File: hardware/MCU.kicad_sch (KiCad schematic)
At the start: 12 parts

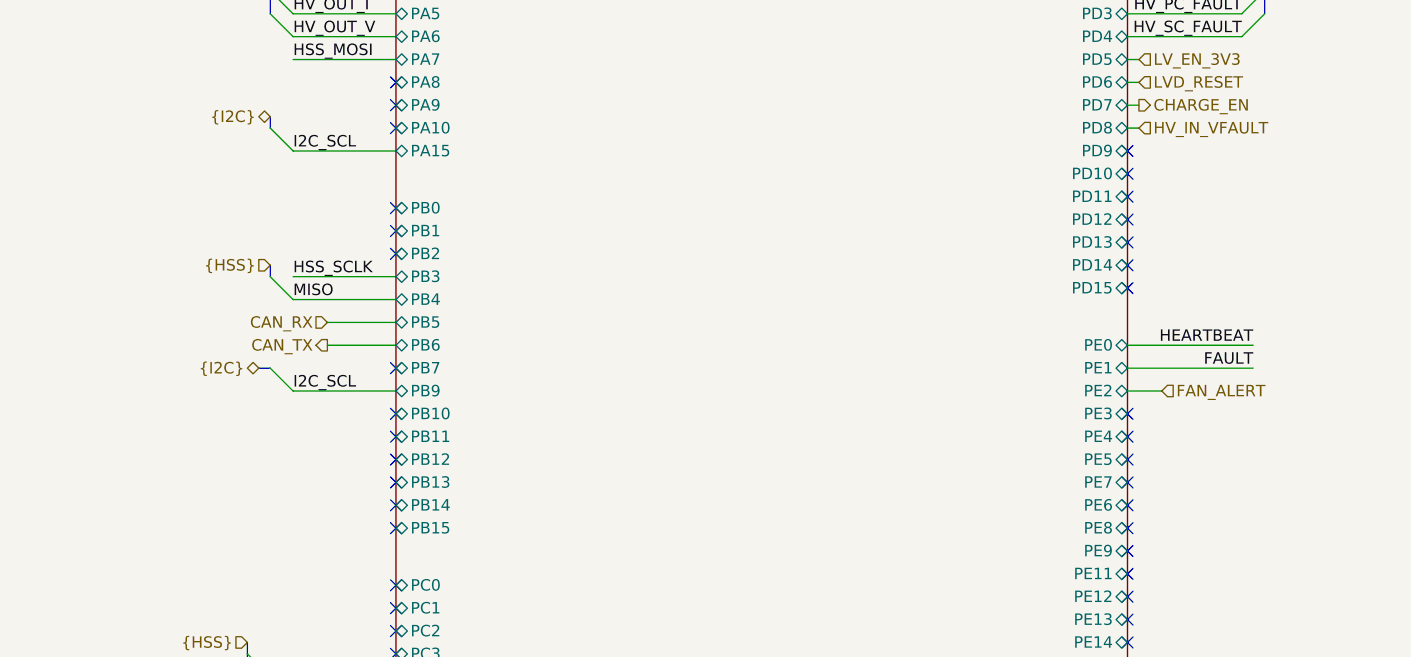
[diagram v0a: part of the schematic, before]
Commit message: review me pt 3
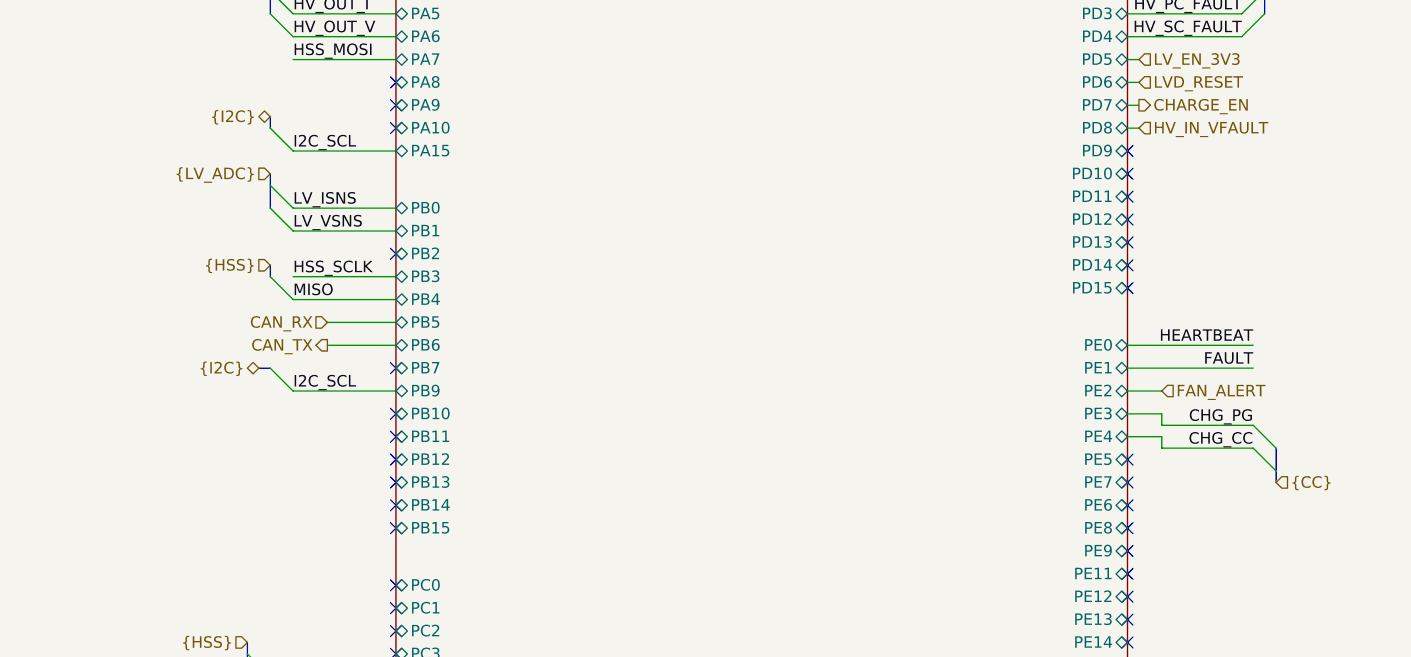
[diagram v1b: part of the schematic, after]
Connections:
- no-connect marks 49 -> 45
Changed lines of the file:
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@@
 	)
 	(no_connect
-		(at 287.02 90.17)
-	)
-	(no_connect
 		(at 287.02 154.94)
 	)
 	(no_connect
-		(at 368.3 110.49)
-	)
-	(no_connect
 		(at 287.02 78.74)
 	)
@@
 	)
 	(no_connect
-		(at 368.3 113.03)
-	)
-	(no_connect
 		(at 368.3 133.35)
 	)
@@
 		(at 368.3 149.86)
 	)
-	(no_connect
-		(at 287.02 87.63)
-	)
 	(bus_entry
 		(at 383.54 63.5)
@@
 	)
 	(bus_entry
+		(at 273.05 85.09)
+		(size 2.54 2.54)
+		(stroke
+			(width 0)
+			(type default)
+		)
+	)
+	(bus_entry
 		(at 273.05 95.25)
 		(size 2.54 2.54)
@@
 	)
 	(bus_entry
+		(at 384.81 114.3)
+		(size -2.54 -2.54)
+		(stroke
+			(width 0)
+			(type default)
+		)
+	)
+	(bus_entry
 		(at 273.05 63.5)
 		(size 2.54 2.54)
@@
 	)
 	(bus_entry
+		(at 273.05 87.63)
+		(size 2.54 2.54)
+		(stroke
+			(width 0)
+			(type default)
+		)
+	)
+	(bus_entry
 		(at 273.05 58.42)
 		(size 2.54 2.54)
@@
 	)
 	(bus_entry
+		(at 384.81 116.84)
+		(size -2.54 -2.54)
+		(stroke
+			(width 0)
+			(type default)
+		)
+	)
+	(bus_entry
 		(at 270.51 137.16)
 		(size 2.54 2.54)
@@
 	(wire
 		(pts
+			(xy 372.11 114.3) (xy 382.27 114.3)
+		)
+		(stroke
+			(width 0)
+			(type default)
+		)
+	)
+	(wire
+		(pts
 			(xy 368.3 73.66) (xy 369.57 73.66)
 		)
@@
 		)
 	)
+	(bus
+		(pts
+			(xy 384.81 114.3) (xy 384.81 118.11)
+		)
+		(stroke
+			(width 0)
+			(type default)
+		)
+	)
 	(wire
 		(pts
@@
 	(wire
 		(pts
+			(xy 275.59 90.17) (xy 287.02 90.17)
+		)
+		(stroke
+			(width 0)
+			(type default)
+		)
+	)
+	(wire
+		(pts
 			(xy 275.59 58.42) (xy 287.02 58.42)
 		)
@@
 	(wire
 		(pts
+			(xy 372.11 110.49) (xy 368.3 110.49)
+		)
+		(stroke
+			(width 0)
+			(type default)
+		)
+	)
+	(wire
+		(pts
 			(xy 287.02 100.33) (xy 279.4 100.33)
 		)
@@
 	(wire
 		(pts
+			(xy 275.59 87.63) (xy 287.02 87.63)
+		)
+		(stroke
+			(width 0)
+			(type default)
+		)
+	)
+	(wire
+		(pts
 			(xy 275.59 50.8) (xy 276.86 50.8)
 		)
@@
 	(wire
 		(pts
+			(xy 372.11 111.76) (xy 372.11 110.49)
+		)
+		(stroke
+			(width 0)
+			(type default)
+		)
+	)
+	(wire
+		(pts
 			(xy 327.66 179.07) (xy 327.66 180.34)
 		)
@@
 	(wire
 		(pts
+			(xy 372.11 113.03) (xy 372.11 114.3)
+		)
+		(stroke
+			(width 0)
+			(type default)
+		)
+	)
+	(wire
+		(pts
 			(xy 275.59 63.5) (xy 287.02 63.5)
 		)
@@
 	(wire
 		(pts
+			(xy 368.3 113.03) (xy 372.11 113.03)
+		)
+		(stroke
+			(width 0)
+			(type default)
+		)
+	)
+	(wire
+		(pts
 			(xy 369.57 78.74) (xy 368.3 78.74)
 		)
@@
 	(bus
 		(pts
+			(xy 273.05 83.82) (xy 273.05 87.63)
+		)
+		(stroke
+			(width 0)
+			(type default)
+		)
+	)
+	(bus
+		(pts
 			(xy 273.05 62.23) (xy 273.05 63.5)
 		)
@@
 	(wire
 		(pts
+			(xy 372.11 111.76) (xy 382.27 111.76)
+		)
+		(stroke
+			(width 0)
+			(type default)
+		)
+	)
+	(wire
+		(pts
 			(xy 292.1 238.76) (xy 289.56 238.76)
 		)
@@
 		)
 	)
+	(label "LV_ISNS"
+		(at 275.59 87.63 0)
+		(effects
+			(font
+				(size 1.27 1.27)
+			)
+			(justify left bottom)
+		)
+	)
 	(label "DI_MODE"
 		(at 273.05 144.78 0)
@@
 		)
 	)
+	(label "CHG_PG"
+		(at 382.27 111.76 180)
+		(effects
+			(font
+				(size 1.27 1.27)
+			)
+			(justify right bottom)
+		)
+	)
 	(label "DI_MODE"
 		(at 316.23 217.17 0)
@@
 		)
 	)
+	(label "LV_VSNS"
+		(at 275.59 90.17 0)
+		(effects
+			(font
+				(size 1.27 1.27)
+			)
+			(justify left bottom)
+		)
+	)
 	(label "USBD+"
 		(at 378.46 52.07 180)
@@
 		)
 	)
+	(label "CHG_CC"
+		(at 382.27 114.3 180)
+		(effects
+			(font
+				(size 1.27 1.27)
+			)
+			(justify right bottom)
+		)
+	)
 	(label "HV_OUT_V"
 		(at 275.59 68.58 0)
@@
 		)
 	)
+	(hierarchical_label "{CC}"
+		(shape input)
+		(at 384.81 118.11 0)
+		(effects
+			(font
+				(size 1.27 1.27)
+			)
+			(justify left)
+		)
+	)
+	(hierarchical_label "{LV_ADC}"
+		(shape input)
+		(at 273.05 83.82 180)
+		(effects
+			(font
+				(size 1.27 1.27)
+			)
+			(justify right)
+		)
+	)
